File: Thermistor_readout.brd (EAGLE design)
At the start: 59.4 x 43.2 mm, 22 parts, among them Q1 BC550C, U1 TI_NATIONAL_SEMICONDUCTOR_LF3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, U2 TI_NATIONAL_SEMICONDUCTOR_LF3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, U3 ANALOG_DEVICES_ADG725BSUZANAL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, U4 TI_NATIONAL_SEMICONDUCTOR_LF3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

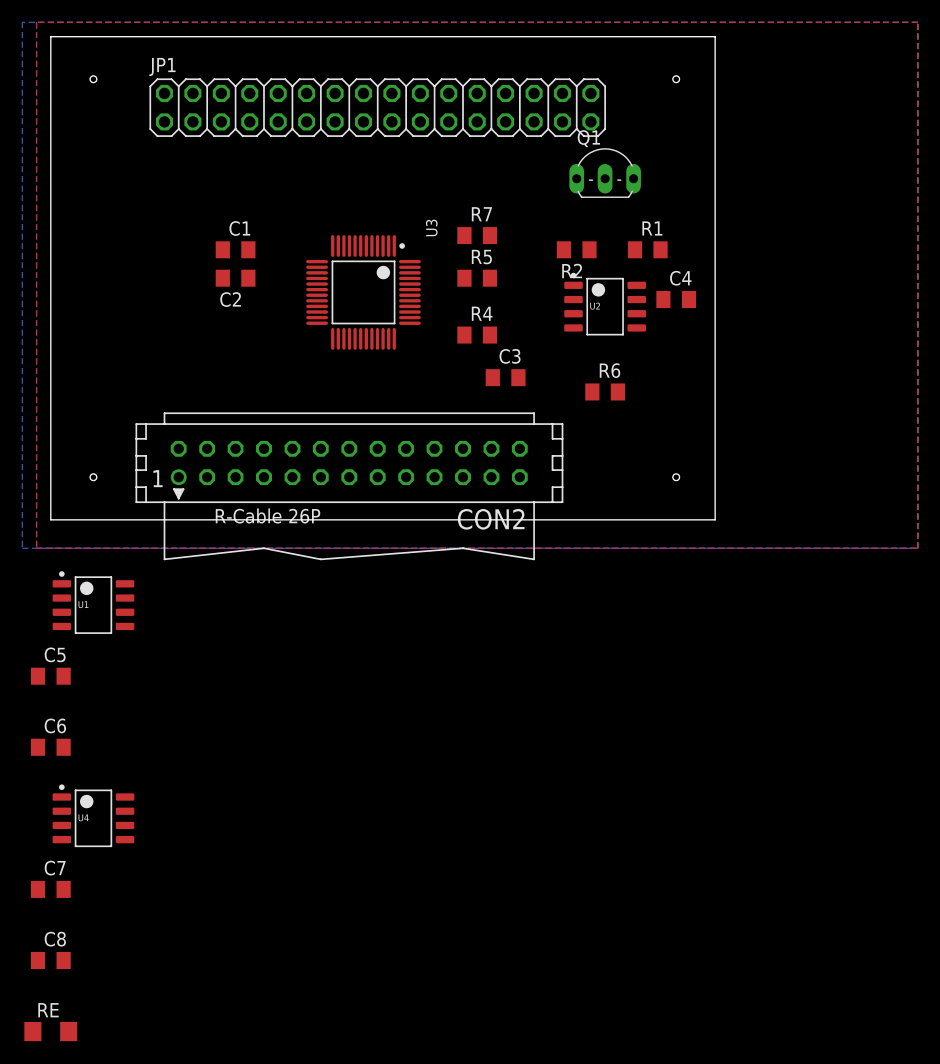
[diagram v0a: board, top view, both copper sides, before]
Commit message: First_PCB_tentative
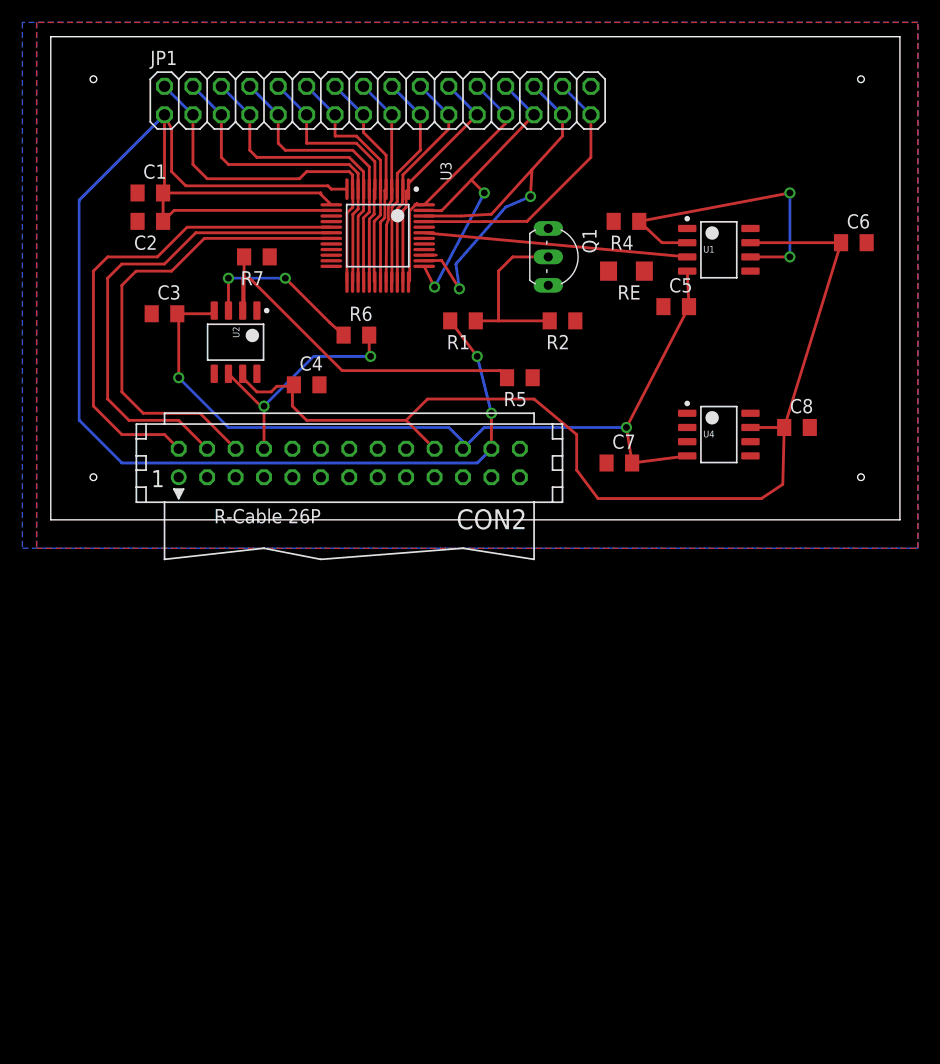
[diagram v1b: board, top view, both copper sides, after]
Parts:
- moved RE 85.2 mm to (51.4, 23.5), turned to 180 degrees
- moved C6 84.7 mm to (71.8, 26.0)
- moved C8 81.9 mm to (66.7, 9.53)
- moved U4 65.6 mm to (59.7, 8.89)
- moved C5 64.9 mm to (55.9, 20.3)
- moved U1 64.3 mm to (59.7, 25.4)
- moved C7 63.5 mm to (50.8, 6.35)
- moved C4 33.9 mm to (22.9, 13.3)
- moved U2 33.2 mm to (16.5, 17.1), turned to 270 degrees
- moved C3 31.0 mm to (10.2, 19.7)
- moved R6 22.8 mm to (27.3, 17.8)
- moved R7 19.8 mm to (18.4, 24.8), turned to 180 degrees
- moved R1 17.7 mm to (36.8, 19.1), turned to 180 degrees
- moved R4 16.8 mm to (51.4, 27.9), turned to 180 degrees
- moved R5 9.67 mm to (41.9, 14.0), turned to 180 degrees
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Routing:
- net +5V: track 0.00 -> 143.9 mm, vias 0 -> 2
- net +15V: track 0.00 -> 95.7 mm
- net -15V: track 0.00 -> 76.5 mm, vias 0 -> 2
- net N$13: track 0.00 -> 44.1 mm
- net N$14: track 0.00 -> 43.2 mm
- net N$11: track 0.00 -> 42.2 mm
- net C$14: track 0.00 -> 39.3 mm, vias 0 -> 2
- net N$5: track 0.00 -> 35.0 mm
- net C$1: track 0.00 -> 33.0 mm
- net C$13: track 0.00 -> 30.3 mm, vias 0 -> 2
- net C$2: track 0.00 -> 30.1 mm
- net N$4: track 0.00 -> 28.0 mm, vias 0 -> 2
- net C$3: track 0.00 -> 27.8 mm
- net C$15: track 0.00 -> 25.8 mm
- net C$4: track 0.00 -> 25.7 mm
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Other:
- board size 59.4 x 43.2 mm -> 75.9 x 43.2 mm
